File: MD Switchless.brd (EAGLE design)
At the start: 20 x 14.6 mm, 13 parts, among them U1 ATTINY85-20S

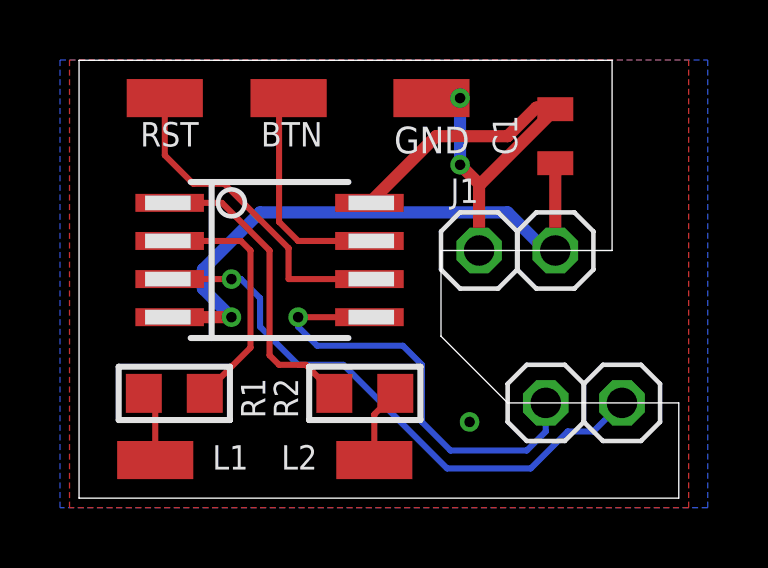
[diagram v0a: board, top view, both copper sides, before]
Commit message: Add files via upload
minor changes
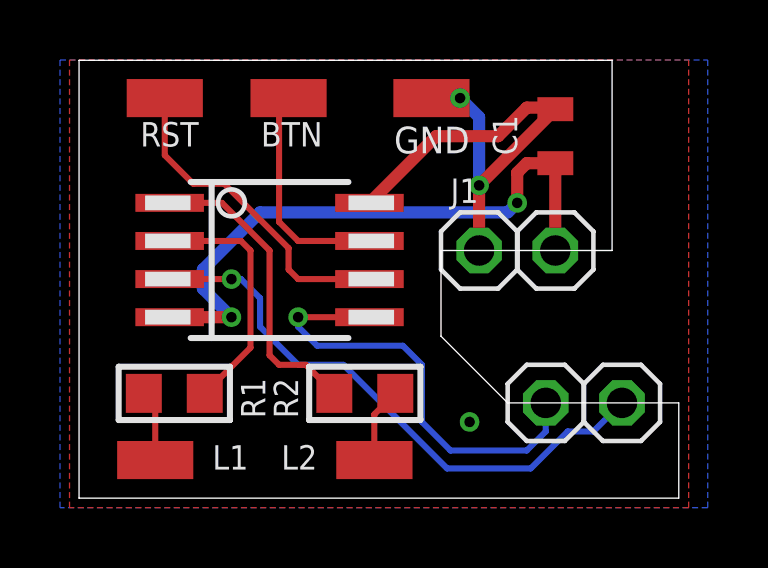
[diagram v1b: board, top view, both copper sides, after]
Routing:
- net 5V: track 20.0 -> 20.8 mm, vias 1 -> 2
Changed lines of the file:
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@@
 <wire x1="9.68" y1="9.8425" x2="11.9025" y2="12.065" width="0.4064" layer="1"/>
 <via x="13.0175" y="2.54" extent="1-16" drill="0.35"/>
-<wire x1="13.335" y1="8.255" x2="13.335" y2="10.425" width="0.4064" layer="1"/>
-<wire x1="13.335" y1="10.425" x2="15.875" y2="12.965" width="0.4064" layer="1"/>
-<wire x1="11.9025" y1="12.065" x2="14.2875" y2="12.065" width="0.4064" layer="1"/>
-<wire x1="14.2875" y1="12.065" x2="15.24" y2="13.0175" width="0.4064" layer="1"/>
-<wire x1="15.24" y1="13.0175" x2="15.8225" y2="13.0175" width="0.4064" layer="1"/>
-<wire x1="15.8225" y1="13.0175" x2="15.875" y2="12.965" width="0.4064" layer="1"/>
-<wire x1="13.335" y1="10.425" x2="13.335" y2="10.4775" width="0.4064" layer="1"/>
-<wire x1="13.335" y1="10.4775" x2="12.7" y2="11.1125" width="0.4064" layer="1"/>
-<via x="12.7" y="11.1125" extent="1-16" drill="0.35"/>
-<wire x1="12.7" y1="11.1125" x2="12.7" y2="13.335" width="0.4064" layer="16"/>
+<wire x1="12.7" y1="13.335" x2="13.335" y2="12.7" width="0.4064" layer="16"/>
 <via x="12.7" y="13.335" extent="1-16" drill="0.35"/>
 <wire x1="12.7" y1="13.335" x2="11.7475" y2="13.335" width="0.4064" layer="1"/>
@@
 <vertex x="-0.635" y="-0.3175"/>
 </polygon>
+<wire x1="15.875" y1="12.965" x2="13.335" y2="10.425" width="0.4064" layer="1"/>
+<wire x1="13.335" y1="10.425" x2="13.335" y2="8.255" width="0.4064" layer="1"/>
+<via x="13.335" y="10.425" extent="1-16" drill="0.35"/>
+<wire x1="13.335" y1="12.7" x2="13.335" y2="10.425" width="0.4064" layer="16"/>
+<wire x1="11.9025" y1="12.065" x2="13.97" y2="12.065" width="0.4064" layer="1"/>
+<wire x1="13.97" y1="12.065" x2="14.9225" y2="13.0175" width="0.4064" layer="1"/>
+<wire x1="14.9225" y1="13.0175" x2="15.8225" y2="13.0175" width="0.4064" layer="1"/>
+<wire x1="15.8225" y1="13.0175" x2="15.875" y2="12.965" width="0.4064" layer="1"/>
+<wire x1="13.0175" y1="2.54" x2="13.335" y2="8.255" width="0" layer="19" extent="1-1"/>
 </signal>
 <signal name="5V" class="2">
@@
 <wire x1="3.02" y1="6.0325" x2="5.08" y2="6.0325" width="0.4064" layer="1"/>
 <via x="5.08" y="6.0325" extent="1-16" drill="0.35"/>
-<wire x1="15.875" y1="8.255" x2="15.5575" y2="8.255" width="0.4064" layer="16"/>
-<wire x1="15.5575" y1="8.255" x2="14.2875" y2="9.525" width="0.4064" layer="16"/>
-<wire x1="14.2875" y1="9.525" x2="6.0325" y2="9.525" width="0.4064" layer="16"/>
+<wire x1="6.0325" y1="9.525" x2="14.2875" y2="9.525" width="0.4064" layer="16"/>
 <wire x1="6.0325" y1="9.525" x2="4.1275" y2="7.62" width="0.4064" layer="16"/>
 <wire x1="4.1275" y1="7.62" x2="4.1275" y2="6.985" width="0.4064" layer="16"/>
 <wire x1="4.1275" y1="6.985" x2="5.08" y2="6.0325" width="0.4064" layer="16"/>
 <wire x1="15.875" y1="8.255" x2="15.875" y2="11.165" width="0.4064" layer="1"/>
+<wire x1="14.2875" y1="9.525" x2="14.605" y2="9.8425" width="0.4064" layer="16"/>
+<via x="14.605" y="9.8425" extent="1-16" drill="0.35"/>
+<wire x1="15.875" y1="11.165" x2="14.9225" y2="11.165" width="0.4064" layer="1"/>
+<wire x1="14.9225" y1="11.165" x2="14.605" y2="10.8475" width="0.4064" layer="1"/>
+<wire x1="14.605" y1="10.8475" x2="14.605" y2="9.8425" width="0.4064" layer="1"/>
 </signal>
 <signal name="LENG">
@@
 <wire x1="2.8575" y1="11.43" x2="3.81" y2="10.4775" width="0.2032" layer="1"/>
 <wire x1="4.8401375" y1="10.4775" x2="6.985" y2="8.3326375" width="0.2032" layer="1"/>
-<wire x1="6.985" y1="8.3326375" x2="6.985" y2="7.3025" width="0.2032" layer="1"/>
-<wire x1="6.985" y1="7.3025" x2="9.68" y2="7.3025" width="0.2032" layer="1"/>
+<wire x1="6.985" y1="8.3326375" x2="6.985" y2="7.62" width="0.2032" layer="1"/>
+<wire x1="6.985" y1="7.62" x2="7.3025" y2="7.3025" width="0.2032" layer="1"/>
+<wire x1="7.3025" y1="7.3025" x2="9.68" y2="7.3025" width="0.2032" layer="1"/>
 <wire x1="3.81" y1="10.4775" x2="4.8401375" y2="10.4775" width="0.2032" layer="1"/>
 </signal>
